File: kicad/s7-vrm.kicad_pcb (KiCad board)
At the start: 2 copper layers, 61.5 x 53 mm, 34 parts, among them J1 Conn_02x15_Row_Letter_First, Q1 Q_NPN_BEC_BRT, Q2 Q_NMOS_GDS, Q3 Q_NMOS_GDS, Q4 Q_PNP_BEC_BRT, SW1 SW_DIP_x04, U1 NCP1579

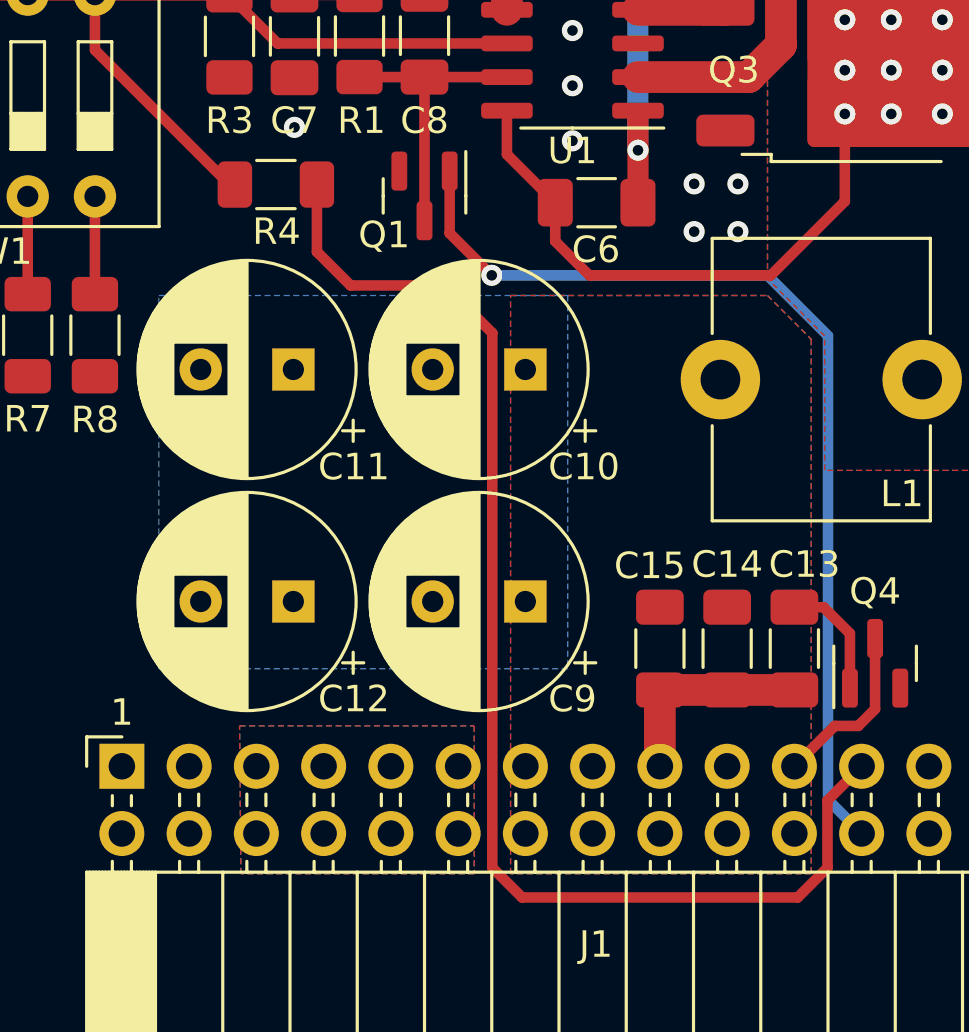
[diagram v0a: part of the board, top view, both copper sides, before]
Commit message: Prepared for production
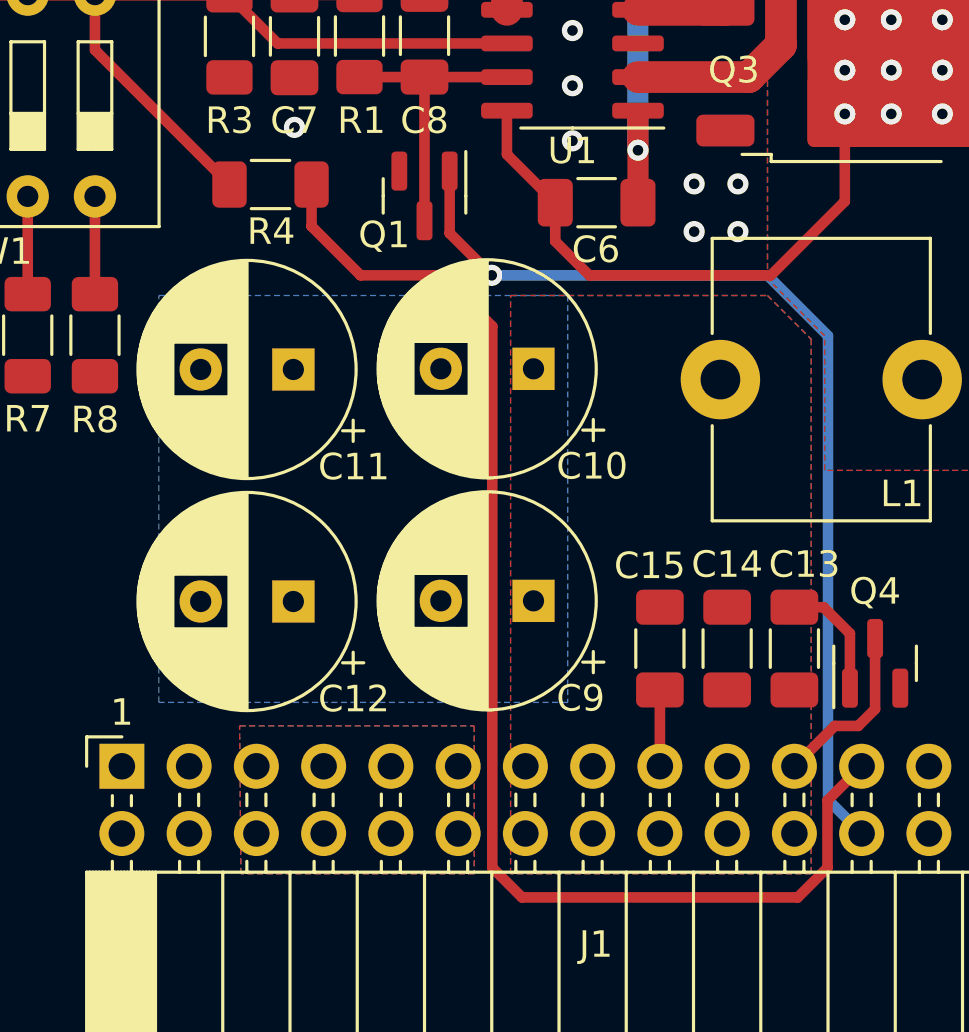
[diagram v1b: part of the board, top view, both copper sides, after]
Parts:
- moved C10 0.31 mm to (147.9, 103.4)
- moved C9 0.31 mm to (147.9, 112.1)
- moved R4 0.20 mm to (137.9, 96.4)
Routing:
- net GND: track 7.84 -> 2.88 mm
